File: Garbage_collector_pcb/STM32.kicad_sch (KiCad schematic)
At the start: 17 parts, among them J2 Conn_ST_STDC14, U3 STM32G431KBTx, Y1 16MHz

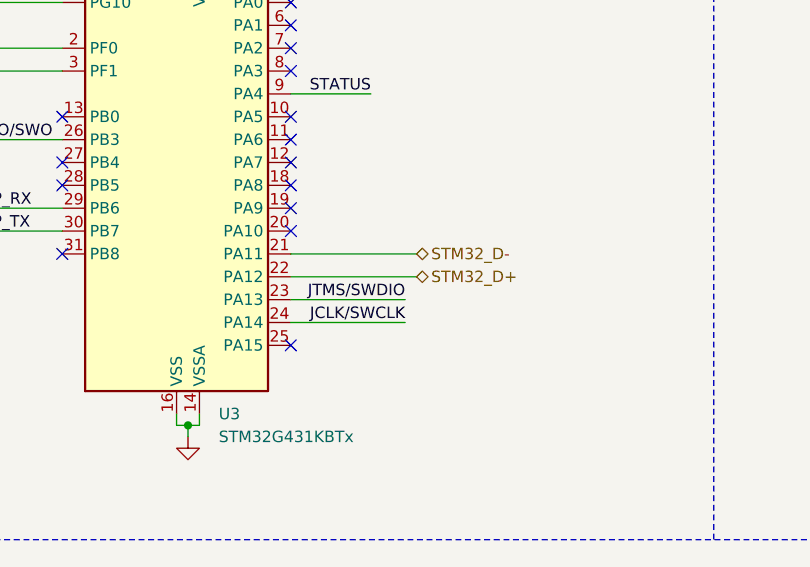
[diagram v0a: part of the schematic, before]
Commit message: Ajout de la partie alimentation
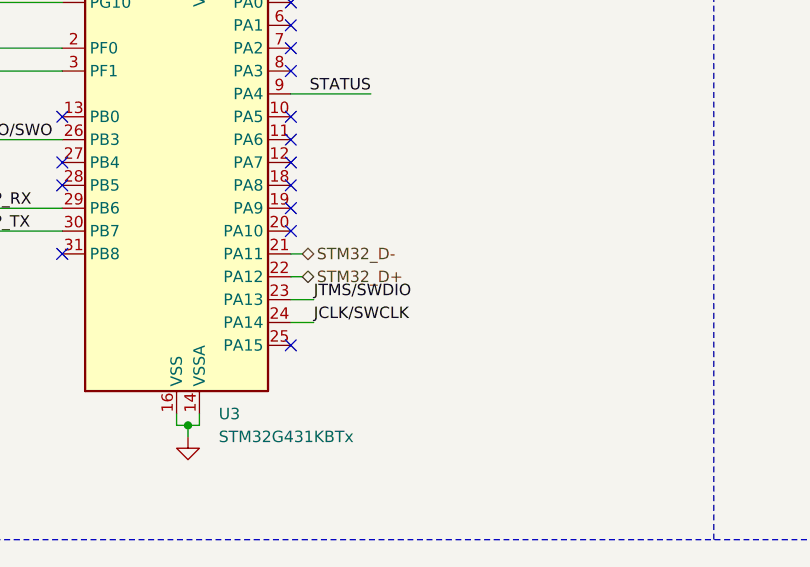
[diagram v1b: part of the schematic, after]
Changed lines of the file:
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@@
 	(wire
 		(pts
-			(xy 125.73 87.63) (xy 111.76 87.63)
+			(xy 113.03 87.63) (xy 111.76 87.63)
 		)
 		(stroke
@@
 	(wire
 		(pts
-			(xy 124.46 95.25) (xy 111.76 95.25)
+			(xy 114.3 95.25) (xy 111.76 95.25)
 		)
 		(stroke
@@
 	(wire
 		(pts
-			(xy 125.73 90.17) (xy 111.76 90.17)
+			(xy 113.03 90.17) (xy 111.76 90.17)
 		)
 		(stroke
@@
 	(wire
 		(pts
-			(xy 124.46 92.71) (xy 111.76 92.71)
+			(xy 114.3 92.71) (xy 111.76 92.71)
 		)
 		(stroke
@@
 	)
 	(label "JTMS/SWDIO"
-		(at 124.46 92.71 180)
-		(effects
-			(font
-				(size 1.27 1.27)
-			)
-			(justify right bottom)
+		(at 114.3 92.71 0)
+		(effects
+			(font
+				(size 1.27 1.27)
+			)
+			(justify left bottom)
 		)
 	)
@@
 	)
 	(label "JCLK/SWCLK"
-		(at 124.46 95.25 180)
-		(effects
-			(font
-				(size 1.27 1.27)
-			)
-			(justify right bottom)
+		(at 114.3 95.25 0)
+		(effects
+			(font
+				(size 1.27 1.27)
+			)
+			(justify left bottom)
 		)
 	)
 	(hierarchical_label "STM32_D+"
 		(shape bidirectional)
-		(at 125.73 90.17 0)
+		(at 113.03 90.17 0)
 		(effects
 			(font
@@
 	(hierarchical_label "STM32_D-"
 		(shape bidirectional)
-		(at 125.73 87.63 0)
-		(effects
-			(font
+		(at 113.03 87.63 0)
+		(effects
+			(font
